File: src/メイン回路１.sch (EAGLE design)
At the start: 18 parts

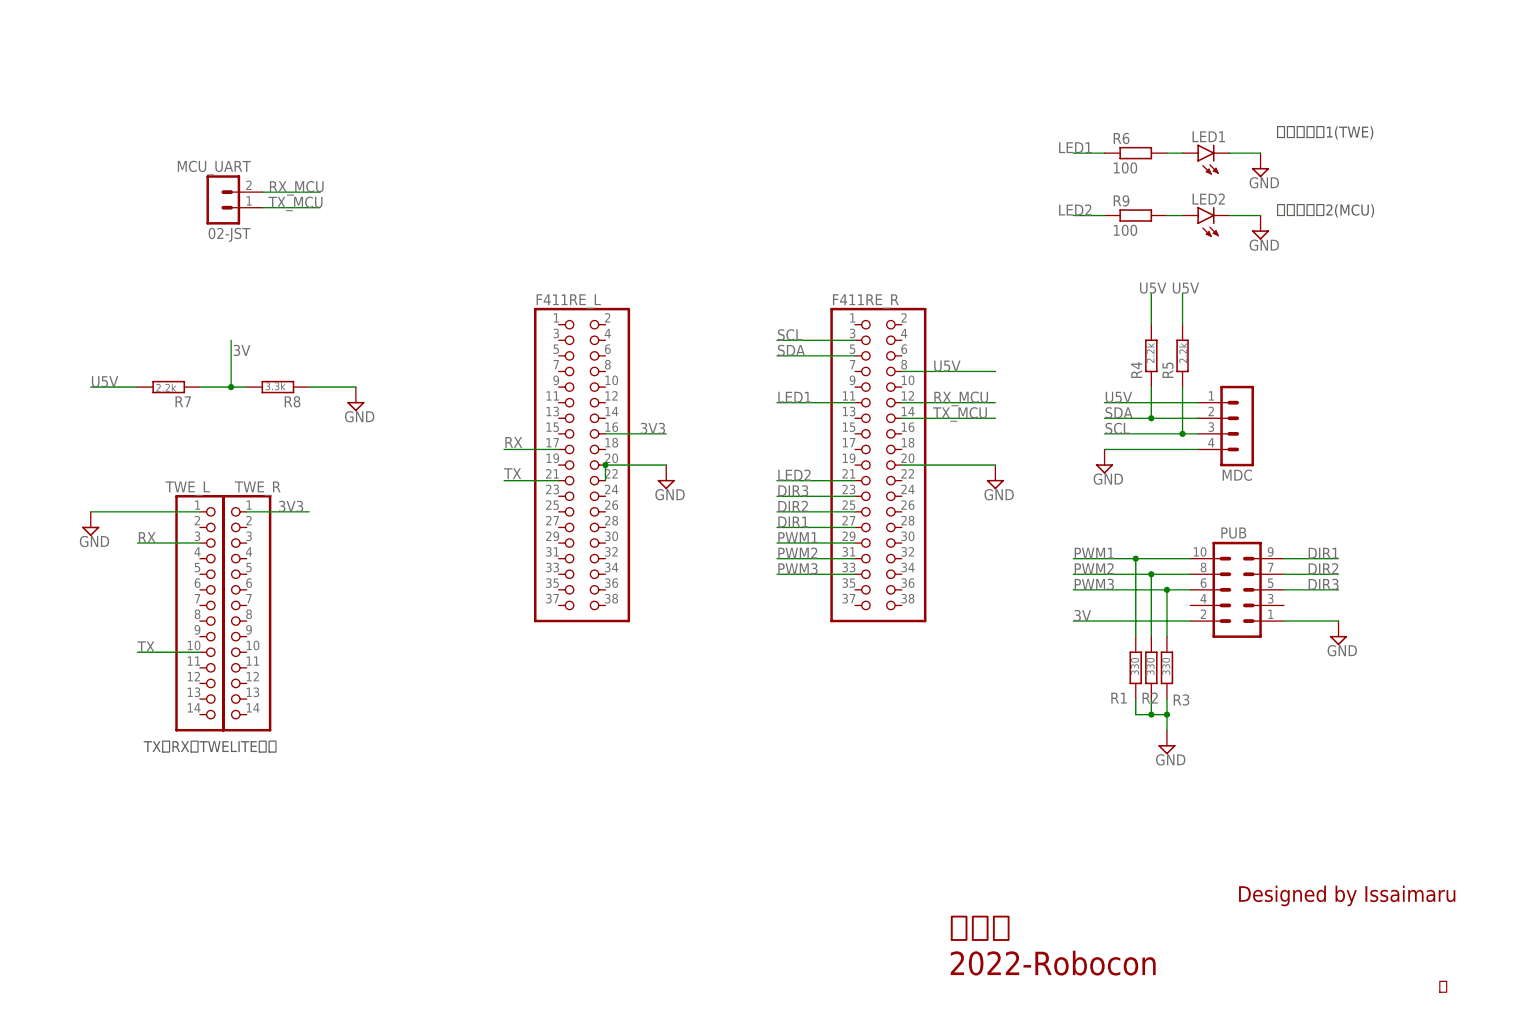
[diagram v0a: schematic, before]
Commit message: [complete]メイン回路1の完成
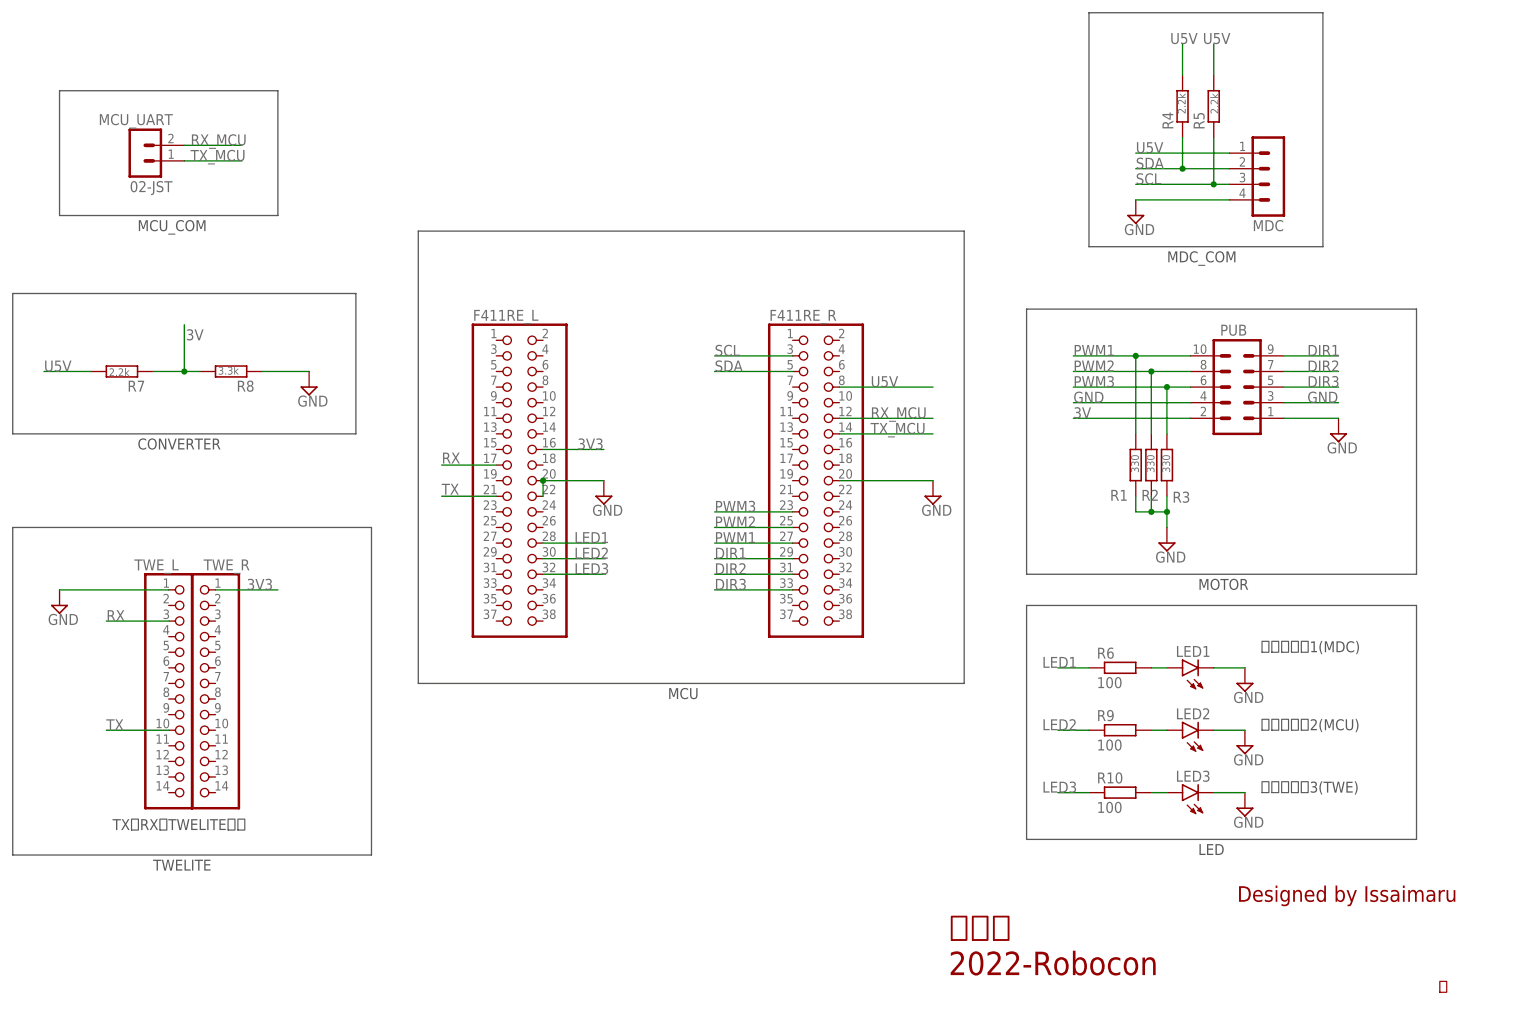
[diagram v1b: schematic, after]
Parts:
- added LED3: (no value), led:LED5MM
- added R10: 100, rcl:R-EU_0204/7
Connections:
- new net LED3: F411RE_L.32, R10.1
- new net N$3: LED3.A, R10.2
- net DIR1: now also F411RE_R.29; no longer F411RE_R.27
- net DIR2: now also F411RE_R.31; no longer F411RE_R.25
- net DIR3: now also F411RE_R.33; no longer F411RE_R.23
- net GND: now also LED3.C, PUB.3, PUB.4
- net LED1: now also F411RE_L.28; no longer F411RE_R.11
- net LED2: now also F411RE_L.30; no longer F411RE_R.21
- net PWM1: now also F411RE_R.27; no longer F411RE_R.29
- net PWM2: now also F411RE_R.25; no longer F411RE_R.31
- net PWM3: now also F411RE_R.23; no longer F411RE_R.33
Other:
- note added: "CONVERTER"
- note added: "LED"
- note added: "MCU"
- note added: "MCU_COM"
- note added: "MDC_COM"
- note added: "MOTOR"
- note added: "TWELITE"
- note added: "受信確認用1(MDC)"
- note added: "受信確認用3(TWE)"
- note removed: "受信確認用1(TWE)"
- moved on the sheet: F411RE_L, F411RE_R, LED1, LED2, MCU_UART, MDC, PUB, R1, R2, R3, R4, R5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
